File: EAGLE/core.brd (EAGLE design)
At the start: 20.3 x 33 mm, 47 parts, among them Q1 MMDT3904, U1 MIC5219, U3 STM32F10XCXT6, U4 SST25VF040B-50-4I-S2AF, X1 USB-MICROB, Y1 8Mhz

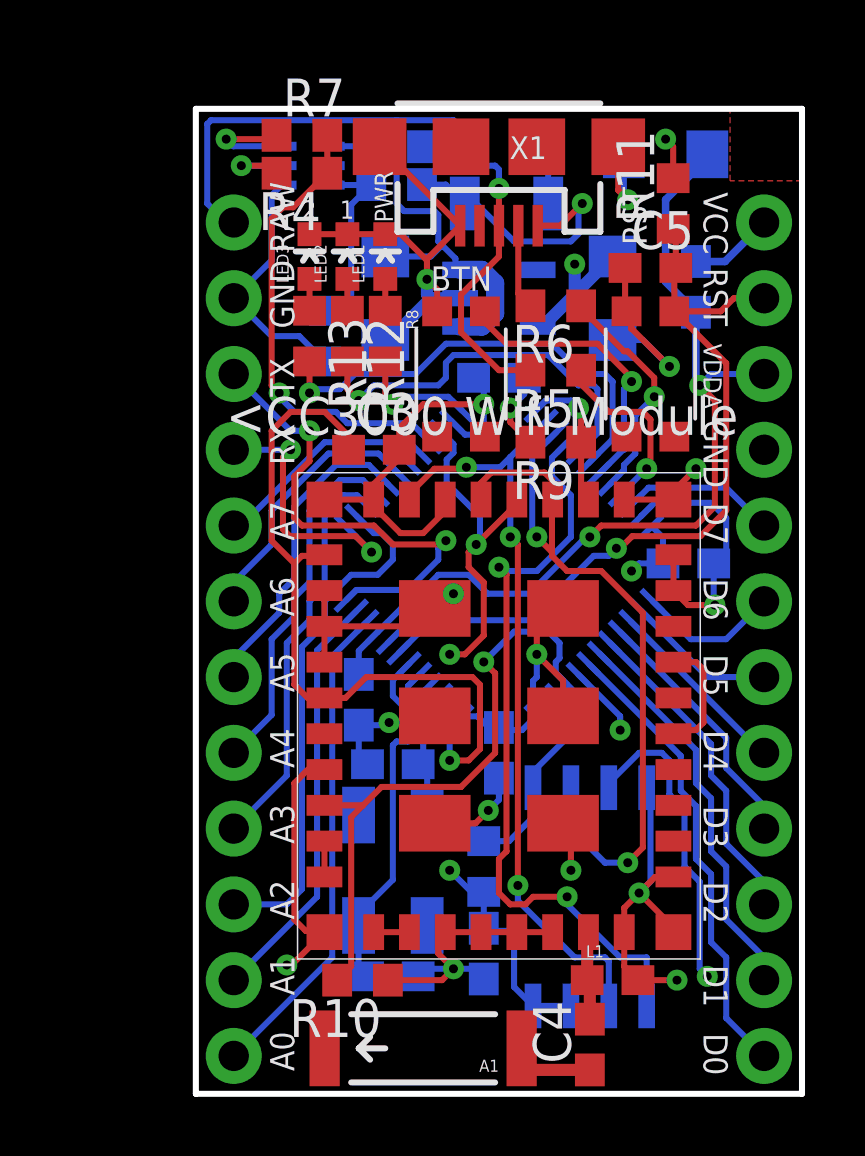
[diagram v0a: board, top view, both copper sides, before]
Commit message: Finished Core Debug v0.0.8
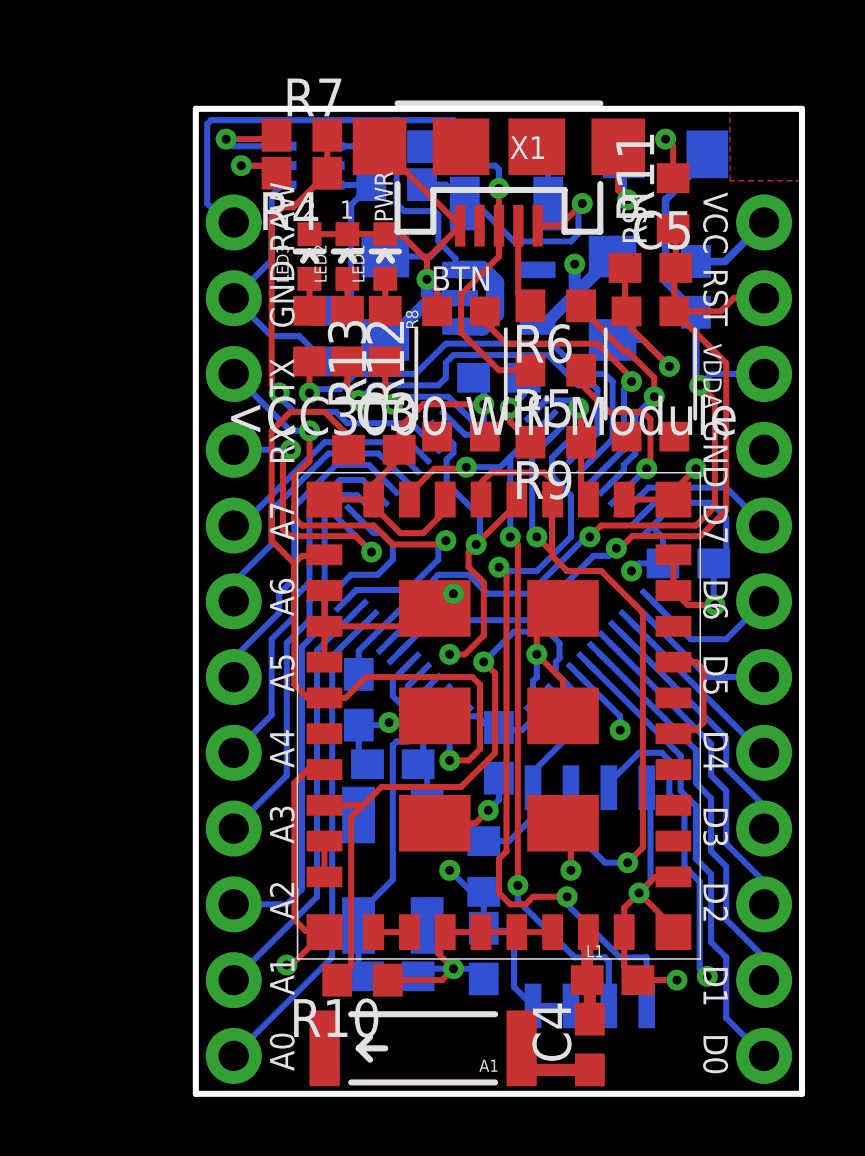
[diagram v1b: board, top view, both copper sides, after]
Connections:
- net SPI_MISO: no longer U2.SPI_DIN
- net SPI_MOSI: now also U2.SPI_DIN
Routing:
- net SPI_MISO: track 27.2 -> 26.7 mm
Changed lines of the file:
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@@
 <setting verticaltext="up"/>
 </settings>
-<grid distance="0.005" unitdist="inch" unit="inch" style="lines" multiple="1" display="yes" altdistance="0.005" altunitdist="inch" altunit="inch"/>
+<grid distance="0.05" unitdist="inch" unit="inch" style="lines" multiple="1" display="yes" altdistance="0.005" altunitdist="inch" altunit="inch"/>
 <layers>
-<layer number="1" name="Top" color="4" fill="1" visible="no" active="yes"/>
+<layer number="1" name="Top" color="4" fill="1" visible="yes" active="yes"/>
 <layer number="2" name="$GND" color="13" fill="1" visible="no" active="yes"/>
 <layer number="3" name="Route3" color="4" fill="3" visible="no" active="no"/>
@@
 <layer number="14" name="Route14" color="1" fill="6" visible="no" active="no"/>
 <layer number="15" name="$+3V3" color="11" fill="1" visible="no" active="yes"/>
-<layer number="16" name="Bottom" color="1" fill="1" visible="no" active="yes"/>
+<layer number="16" name="Bottom" color="1" fill="1" visible="yes" active="yes"/>
 <layer number="17" name="Pads" color="2" fill="1" visible="yes" active="yes"/>
-<layer number="18" name="Vias" color="2" fill="1" visible="no" active="yes"/>
-<layer number="19" name="Unrouted" color="6" fill="1" visible="no" active="yes"/>
+<layer number="18" name="Vias" color="2" fill="1" visible="yes" active="yes"/>
+<layer number="19" name="Unrouted" color="6" fill="1" visible="yes" active="yes"/>
 <layer number="20" name="Dimension" color="6" fill="1" visible="yes" active="yes"/>
 <layer number="21" name="tPlace" color="16" fill="1" visible="yes" active="yes"/>
-<layer number="22" name="bPlace" color="14" fill="1" visible="no" active="yes"/>
+<layer number="22" name="bPlace" color="14" fill="1" visible="yes" active="yes"/>
 <layer number="23" name="tOrigins" color="15" fill="1" visible="yes" active="yes"/>
-<layer number="24" name="bOrigins" color="15" fill="1" visible="no" active="yes"/>
+<layer number="24" name="bOrigins" color="15" fill="1" visible="yes" active="yes"/>
 <layer number="25" name="tNames" color="7" fill="1" visible="no" active="yes"/>
 <layer number="26" name="bNames" color="7" fill="1" visible="no" active="yes"/>
-<layer number="27" name="tValues" color="7" fill="1" visible="yes" active="yes"/>
+<layer number="27" name="tValues" color="7" fill="1" visible="no" active="yes"/>
 <layer number="28" name="bValues" color="7" fill="1" visible="no" active="yes"/>
 <layer number="29" name="tStop" color="7" fill="3" visible="no" active="yes"/>
 <layer number="30" name="bStop" color="7" fill="6" visible="no" active="yes"/>
-<layer number="31" name="tCream" color="7" fill="4" visible="yes" active="yes"/>
+<layer number="31" name="tCream" color="7" fill="4" visible="no" active="yes"/>
 <layer number="32" name="bCream" color="7" fill="5" visible="no" active="yes"/>
 <layer number="33" name="tFinish" color="6" fill="3" visible="no" active="yes"/>
@@
 <signal name="SPI_MISO">
 <contactref element="U2" pad="SPI_DOUT"/>
-<contactref element="U2" pad="SPI_DIN"/>
 <contactref element="U3" pad="27"/>
 <contactref element="U4" pad="2"/>
@@
 <wire x1="11.938" y1="18.034" x2="11.938" y2="18.161" width="0.2032" layer="1"/>
 <wire x1="11.938" y1="18.161" x2="11.43" y2="18.669" width="0.2032" layer="1"/>
-<wire x1="9.56" y1="19.92" x2="9.56" y2="20.482" width="0.2032" layer="1"/>
 <wire x1="9.56" y1="20.482" x2="9.906" y2="20.828" width="0.2032" layer="1"/>
 <wire x1="9.906" y1="20.828" x2="11.684" y2="20.828" width="0.2032" layer="1"/>
@@
 <wire x1="10.16" y1="17.653" x2="10.287" y2="17.526" width="0.2032" layer="16"/>
 <wire x1="10.287" y1="17.526" x2="11.43" y2="17.526" width="0.2032" layer="16"/>
+<contactref element="U2" pad="SPI_DIN"/>
+<wire x1="10.16" y1="17.653" x2="9.56" y2="19.92" width="0" layer="19" extent="1-16"/>
 </signal>
 <signal name="USB_DISC">
